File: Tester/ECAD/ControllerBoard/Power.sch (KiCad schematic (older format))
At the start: 15 parts, among them U6 TPS2046B, U7 TLV70033_SOT23-5, U8 TLV70033_SOT23-5

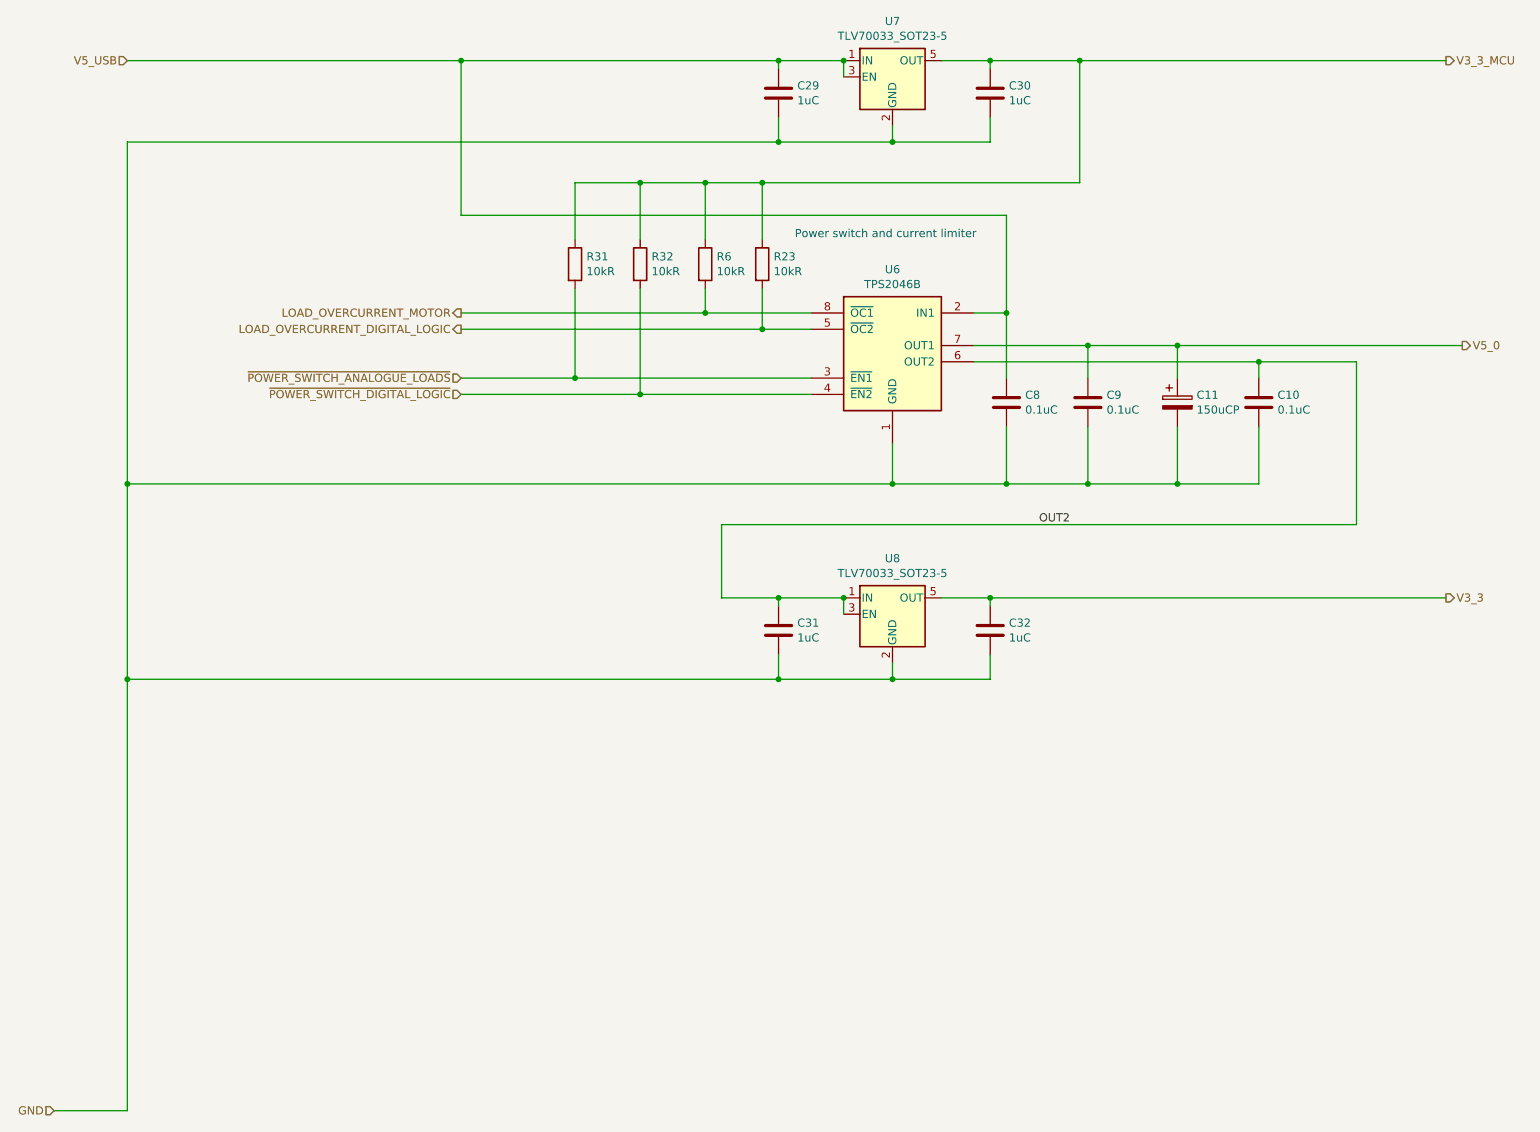
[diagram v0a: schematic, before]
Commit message: Progressed circuit updates.
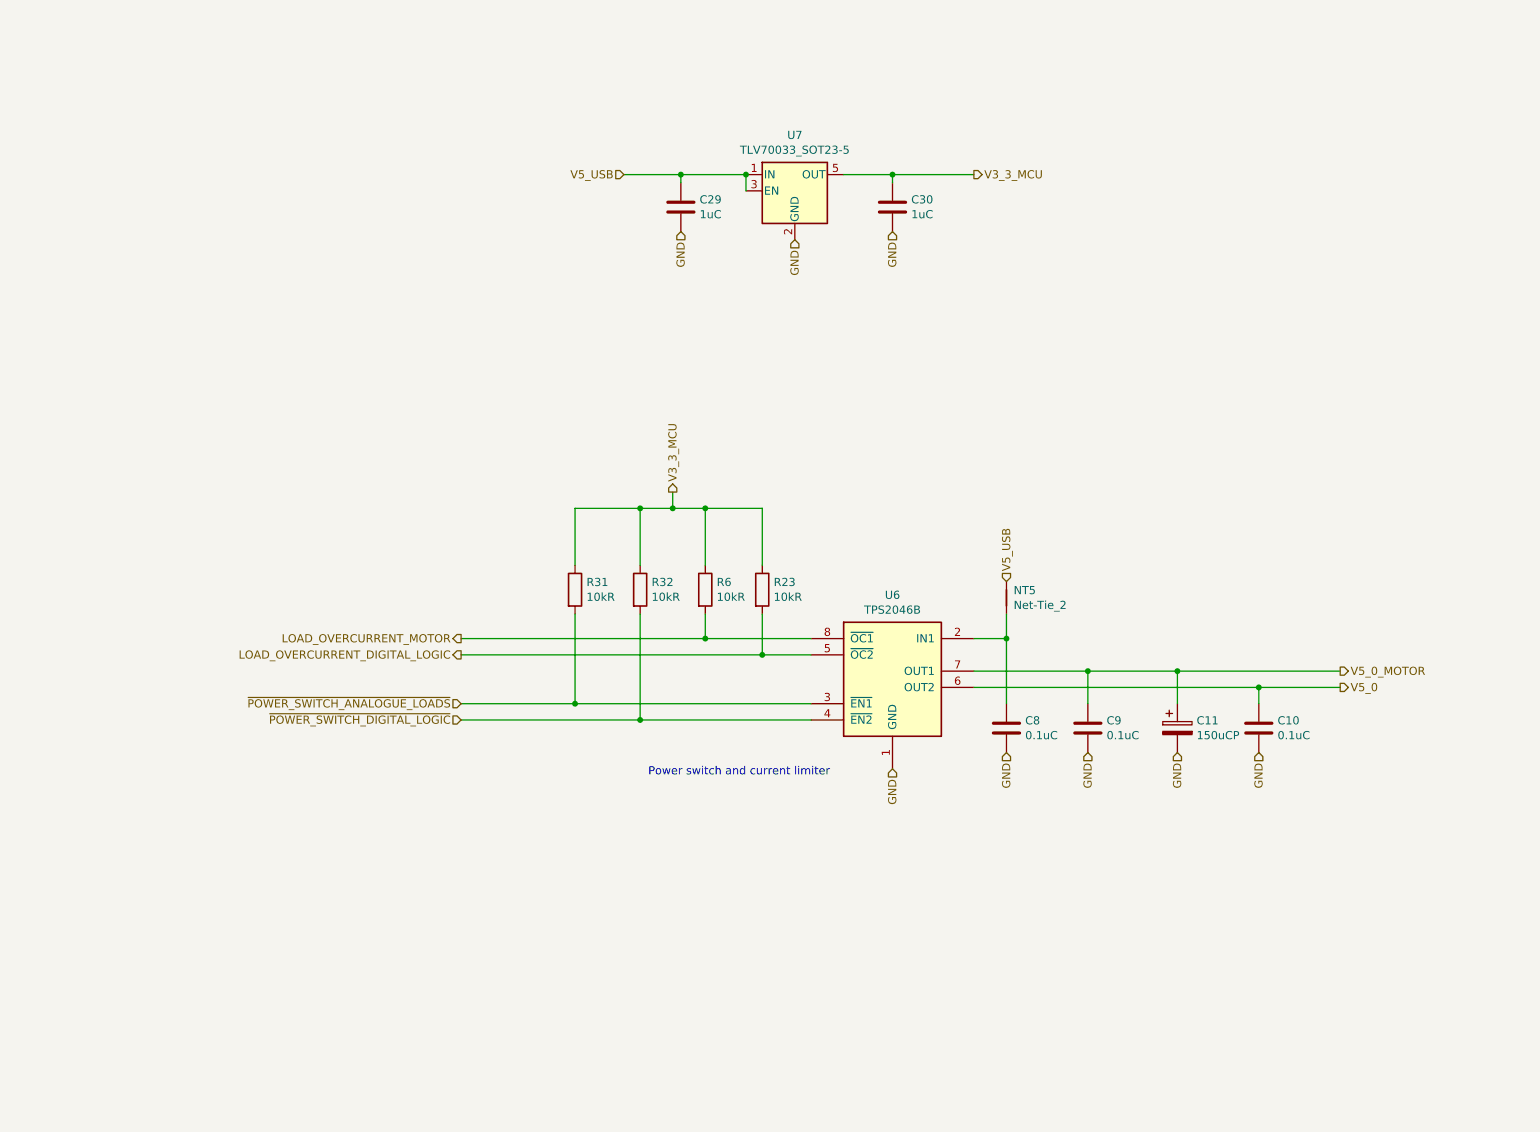
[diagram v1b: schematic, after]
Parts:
- removed C31, C32: 1uC, Capacitor_SMD:C_0805_2012Metric_Pad1.15x1.40mm_HandSolder, symbol Device:C
- removed U8: TLV70033_SOT23-5, Package_TO_SOT_SMD:SOT-23-5, symbol Regulator_Linear:TLV70033_SOT23-5
- added NT5: Net-Tie_2, symbol Device:Net-Tie_2
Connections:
- net OUT2 is gone; now on net V5_0: C10.1, U6.6 (OUT2)
- net V5_0: no longer C11.1, C9.1, U6.7 (OUT1)
- net V5_USB: now also NT5.1; no longer C8.1, U6.2 (IN1)
- new net: C8.1, NT5.2, U6.2 (IN1)
- new net V5_0_MOTOR: C11.1, C9.1, U6.7 (OUT1)
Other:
- moved on the sheet: C10, C11, C29, C30, C8, C9, R23, R31, R32, R6, U6, U7
